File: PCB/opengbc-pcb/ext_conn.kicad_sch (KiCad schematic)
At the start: 13 parts, among them P3 EXT_CONNECTOR

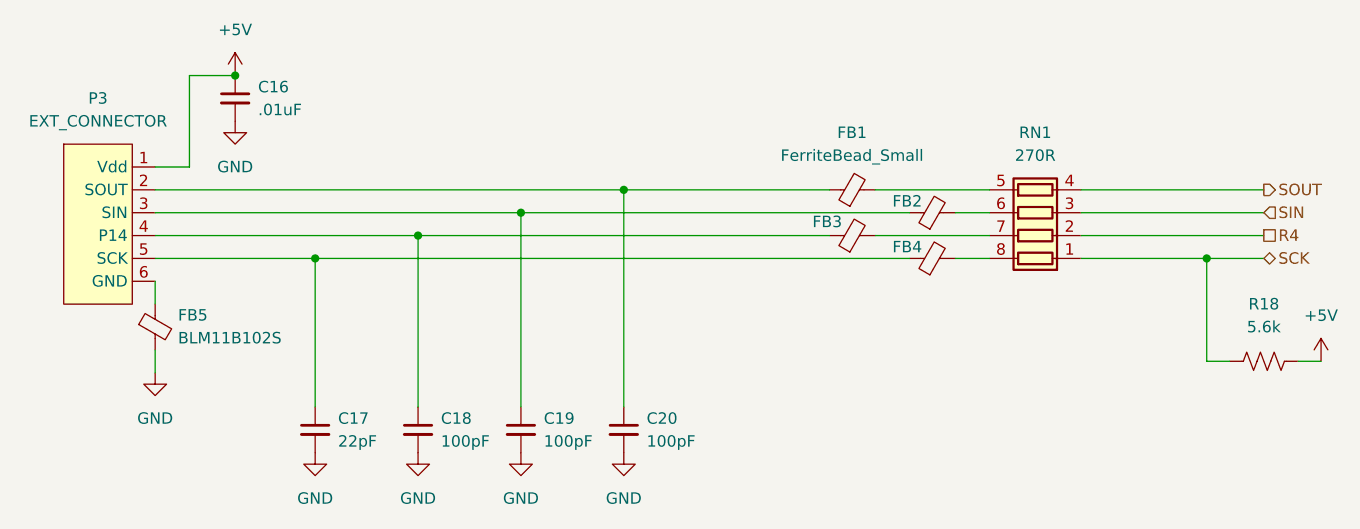
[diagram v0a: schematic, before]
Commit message: :eyes:
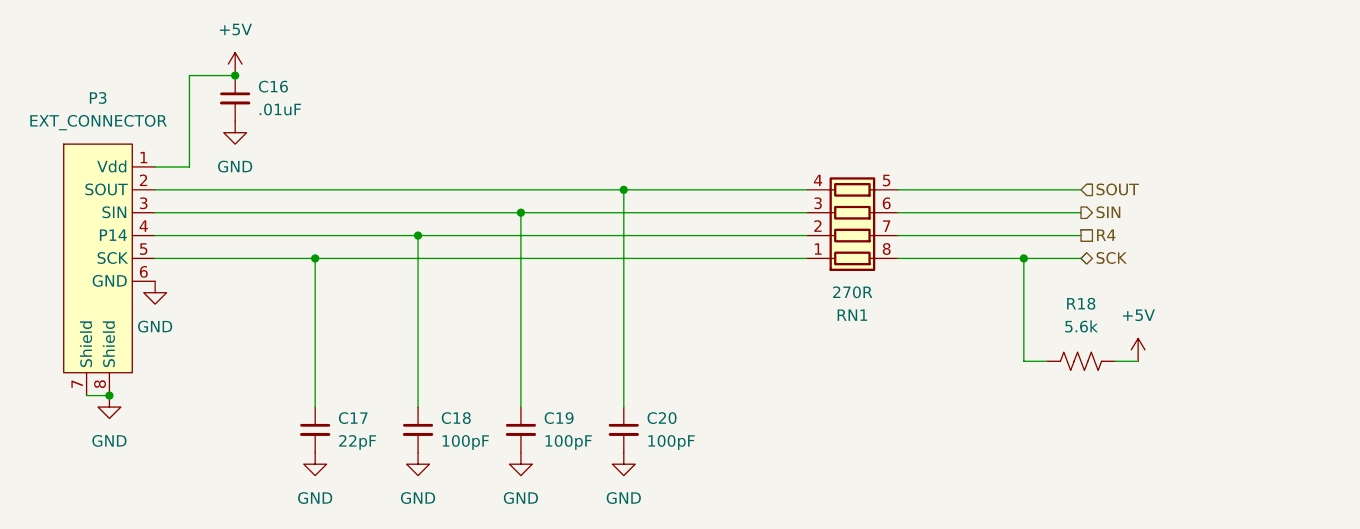
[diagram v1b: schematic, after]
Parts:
- removed FB1, FB2, FB3, FB4: FerriteBead_Small, symbol Device:FerriteBead_Small
- removed FB5: BLM11B102S, symbol Device:FerriteBead_Small
- C16: footprint (none) -> Capacitor_SMD:C_0603_1608Metric_Pad1.08x0.95mm_HandSolder; Mouser Part Number (none) -> 81-GRT188R72A103KE1D
- C17: footprint (none) -> Capacitor_SMD:C_0603_1608Metric_Pad1.08x0.95mm_HandSolder; Mouser Part Number (none) -> 810-C1608C0G1H220J
- C18, C19, C20: footprint (none) -> Capacitor_SMD:C_0603_1608Metric_Pad1.08x0.95mm_HandSolder; Mouser Part Number (none) -> 77-VJ0603Y101MXACBC
- P3: footprint (none) -> link-port:gbc-link-cable-adapter; now left out of the parts list
- R18: footprint (none) -> Resistor_SMD:R_0603_1608Metric_Pad0.98x0.95mm_HandSolder; Mouser Part Number (none) -> 71-CRCW06035K60FKEAC
- RN1: footprint (none) -> Resistor_SMD:R_Array_Concave_4x0603; Mouser Part Number (none) -> 603-AC0603FR-07270RL
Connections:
- net GND: now also P3.6 (GND), P3.7 (Shield), P3.8 (Shield)
- net R4: now also RN1.7 (R2.2); no longer RN1.2 (R2.1)
- net SCK: now also RN1.8 (R1.2); no longer RN1.1 (R1.1)
- net SIN: now also RN1.6 (R3.2); no longer RN1.3 (R3.1)
- net SOUT: now also RN1.5 (R4.2); no longer RN1.4 (R4.1)
- net at C17.1, P3.5 (SCK): now also RN1.1 (R1.1)
- net at C19.1, P3.3 (SIN): now also RN1.3 (R3.1)
- net at C20.1, P3.2 (SOUT): now also RN1.4 (R4.1)
- net at C18.1, P3.4 (P14): now also RN1.2 (R2.1)
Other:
- moved on the sheet: R18, RN1
